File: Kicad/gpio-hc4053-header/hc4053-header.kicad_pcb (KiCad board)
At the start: 2 copper layers, 50 x 25 mm, 10 parts, among them K1 GPIO IN, K3 I/O, K4 I/O, U1 74HC4053, U2 3M-SJ5376

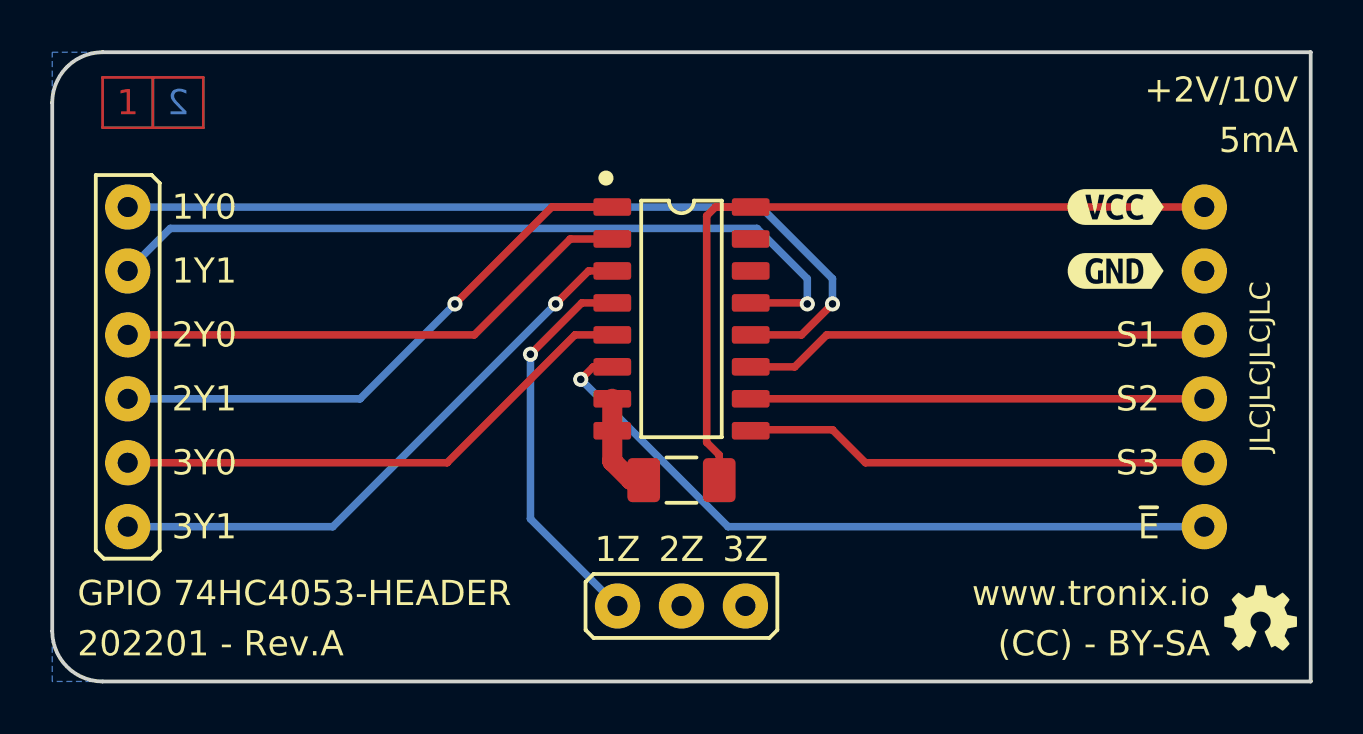
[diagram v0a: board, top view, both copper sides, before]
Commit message: Update
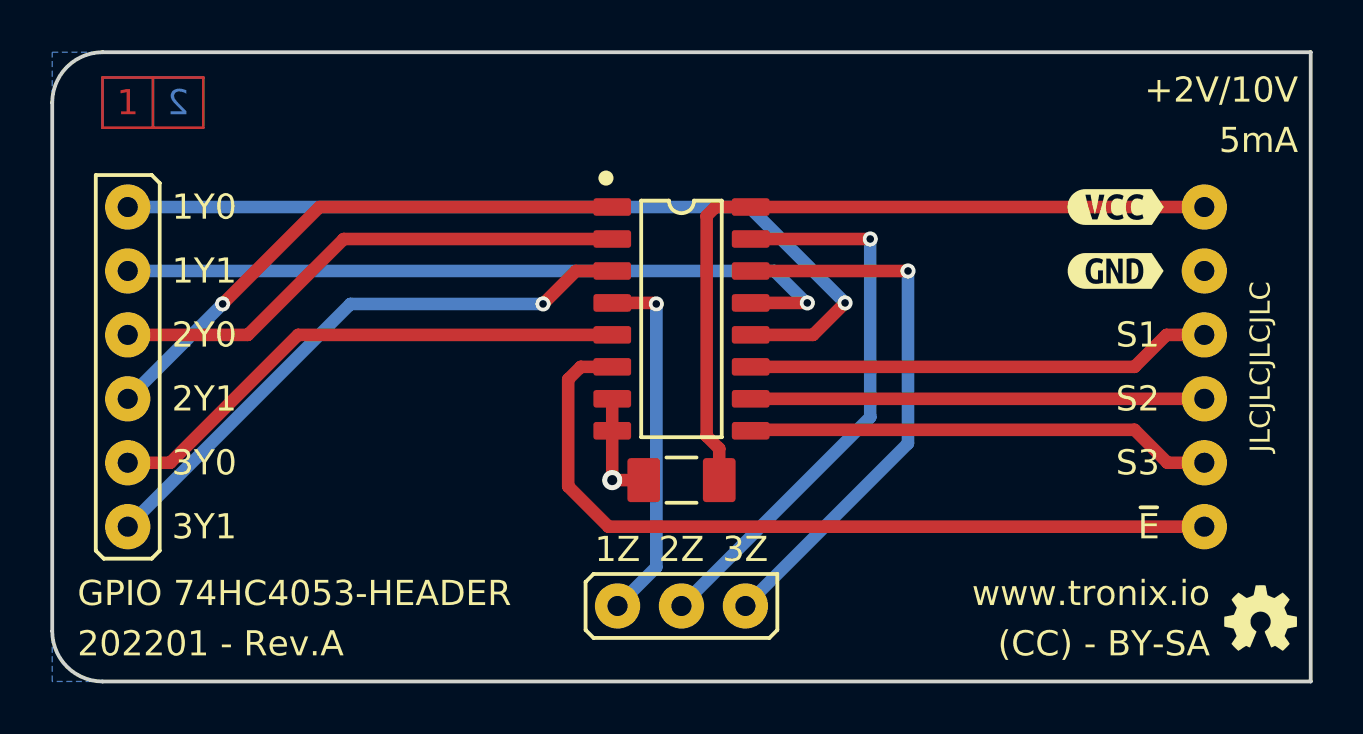
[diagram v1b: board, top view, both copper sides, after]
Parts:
- C1: footprint tronixio:CAPACITOR-1206 -> tronixio:CAPACITOR-SMD-1206
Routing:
- net Net-(K3-Pad2): track 0.00 -> 22.4 mm, vias 0 -> 1
- net Net-(K3-Pad1): track 0.00 -> 22.2 mm, vias 0 -> 1
- net Net-(K1-Pad6): track 28.7 -> 32.1 mm, vias 1 -> 0
- net Net-(K4-Pad2): track 31.8 -> 29.8 mm
- net Net-(K3-Pad3): track 15.5 -> 14.4 mm
- net GND: track 4.04 -> 4.48 mm, vias 0 -> 1
